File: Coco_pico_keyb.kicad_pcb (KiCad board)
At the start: 2 copper layers, 65.5 x 70.5 mm, 13 parts, among them J1 Conn_01x16_Pin, J2 DE9_Plug_MountingHoles, J3 Conn_01x16_Pin, U1 Pico

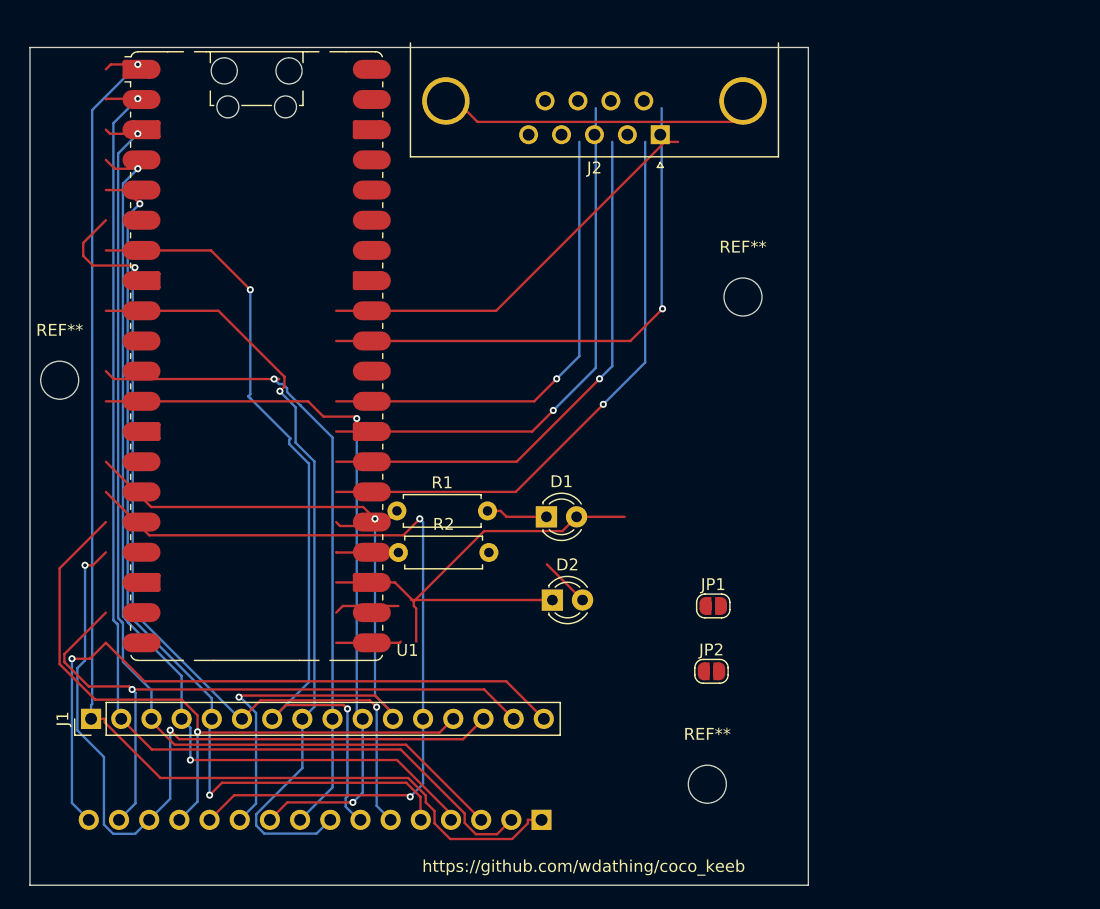
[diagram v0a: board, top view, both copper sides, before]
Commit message: Update board layout
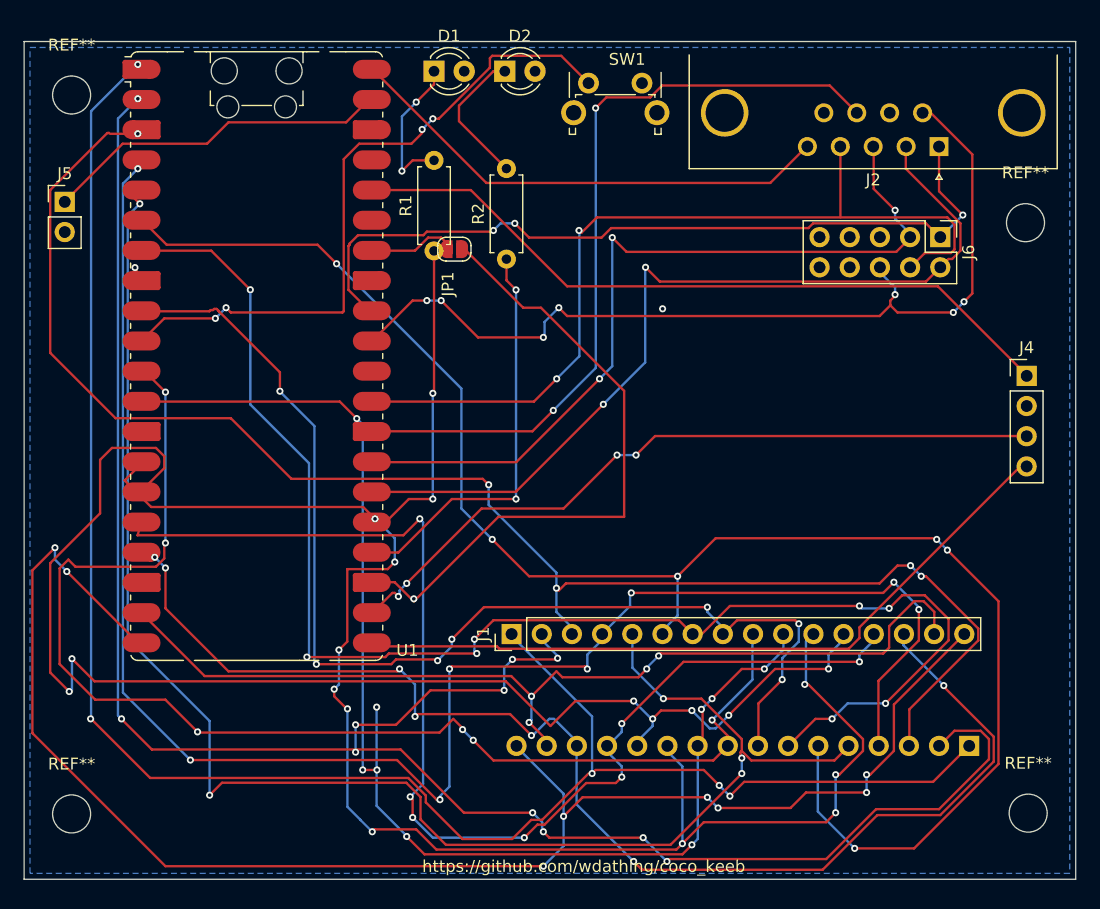
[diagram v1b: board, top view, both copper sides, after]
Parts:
- removed JP2: OPEN=HOST, Jumper:SolderJumper-2_P1.3mm_Open_RoundedPad1.0x1.5mm
- removed the REF** at (139.5, 49.0)
- added J4: SSD1306 I2C Display (optional), Connector_PinHeader_2.54mm:PinHeader_1x04_P2.54mm_Vertical, F.Cu at (163.4, 55.6)
- added J5: Power In, Connector_PinHeader_2.54mm:PinHeader_1x02_P2.54mm_Vertical, F.Cu at (82.4, 41.0)
- added J6: Remote DE9, Connector_PinHeader_2.54mm:PinHeader_2x05_P2.54mm_Vertical, F.Cu at (156.1, 44.0)
- added REF**: MountingHole_3.2mm_M3, MountingHole:MountingHole_3.2mm_M3, F.Cu at (163.3, 42.7)
- added REF**: MountingHole_3.2mm_M3, MountingHole:MountingHole_3.2mm_M3, F.Cu at (163.5, 92.4)
- added SW1: Pairing Button, Button_Switch_THT:SW_Tactile_SPST_Angled_PTS645Vx39-2LFS, F.Cu at (126.5, 31.0)
- moved REF** 53.6 mm to (83.0, 92.5)
- moved D2 44.7 mm to (119.5, 30.0)
- moved D1 38.7 mm to (113.5, 30.0)
- moved JP1 37.1 mm to (115.2, 45.0)
- moved J3 36.5 mm to (158.5, 86.8)
- moved J1 36.1 mm to (120.0, 77.4)
- moved R2 26.3 mm to (119.6, 45.8), turned to 90 degrees
- moved REF** 24.0 mm to (83.0, 32.0)
- moved J2 23.5 mm to (156.0, 36.3)
- moved R1 22.1 mm to (113.5, 45.1), turned to 90 degrees
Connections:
- net Net-(D1-A) renamed /GND
- net Net-(U1-GPIO20) renamed /GPIO20
- net Net-(U1-GPIO21) renamed /GPIO21
- net Net-(U1-GPIO22) renamed /GPIO22
- net Net-(U1-GPIO26_ADC0) renamed /GPIO26_ADC0
- net Net-(U1-GPIO27_ADC1) renamed /GPIO27_ADC1
- J2 pad 5: unconnected-(J2-Pad5) -> Net-(U1-VBUS)
- JP1 pad 1: Net-(JP1-A) -> /DRAGON_SEL
- U1 pad 10: unconnected-(U1-GPIO7-Pad10) -> /BTN_PAIR
- U1 pad 21: Net-(JP2-A) -> /I2C0_SDA
- U1 pad 22: Net-(JP1-A) -> /I2C0_SCL
- U1 pad 34: unconnected-(U1-GPIO28_ADC2-Pad34) -> /DRAGON_SEL
- U1 pad 36: unconnected-(U1-3V3-Pad36) -> /3V3
- U1 pad 39: unconnected-(U1-VSYS-Pad39) -> /VSYS
- U1 pad 40: unconnected-(U1-VBUS-Pad40) -> Net-(U1-VBUS)
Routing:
- net Net-(J1-Pin_16): track 57.1 -> 131.3 mm, vias 1 -> 8
- net Net-(J1-Pin_2): track 94.1 -> 166.1 mm, vias 1 -> 11
- net Net-(J1-Pin_6): track 72.7 -> 137.6 mm, vias 2 -> 6
- net Net-(J1-Pin_4): track 80.4 -> 144.1 mm, vias 2 -> 8
- net /I2C0_SCL: track 0.00 -> 61.6 mm, vias 0 -> 4
- net /3V3: track 0.00 -> 61.6 mm
- net /I2C0_SDA: track 0.00 -> 61.1 mm
- net Net-(J1-Pin_11): track 67.7 -> 124.5 mm, vias 2 -> 10
- net /BTN_PAIR: track 0.00 -> 56.7 mm, vias 0 -> 4
- net Net-(J1-Pin_5): track 77.2 -> 132.7 mm, vias 2 -> 5
- net Net-(J1-Pin_1): track 103.6 -> 154.3 mm, vias 1 -> 5
- net Net-(J1-Pin_7): track 70.4 -> 121.0 mm, vias 2 -> 8
- net Net-(J1-Pin_9): track 56.5 -> 106.6 mm, vias 1 -> 6
- net Net-(J1-Pin_10): track 62.2 -> 107.5 mm, vias 2 -> 9
- net Net-(J1-Pin_3): track 85.6 -> 130.3 mm, vias 1 -> 5
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- added copper zone on B.Cu, net /GND
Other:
- board size 65.5 x 70.5 mm -> 88.5 x 70.5 mm
